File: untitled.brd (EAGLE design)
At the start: 92.9 x 80 mm, 176 parts, among them IC1 MCP23017SS, IC4 MCP23017SS, K2 351, Q1 S9013, U49 PC817X2NIP0F, X1 MSTBA12, X2 MSTBA12, X5 MSTBA3, X6 MSTBA3, X7 MSTBA2, X8 MSTBA2

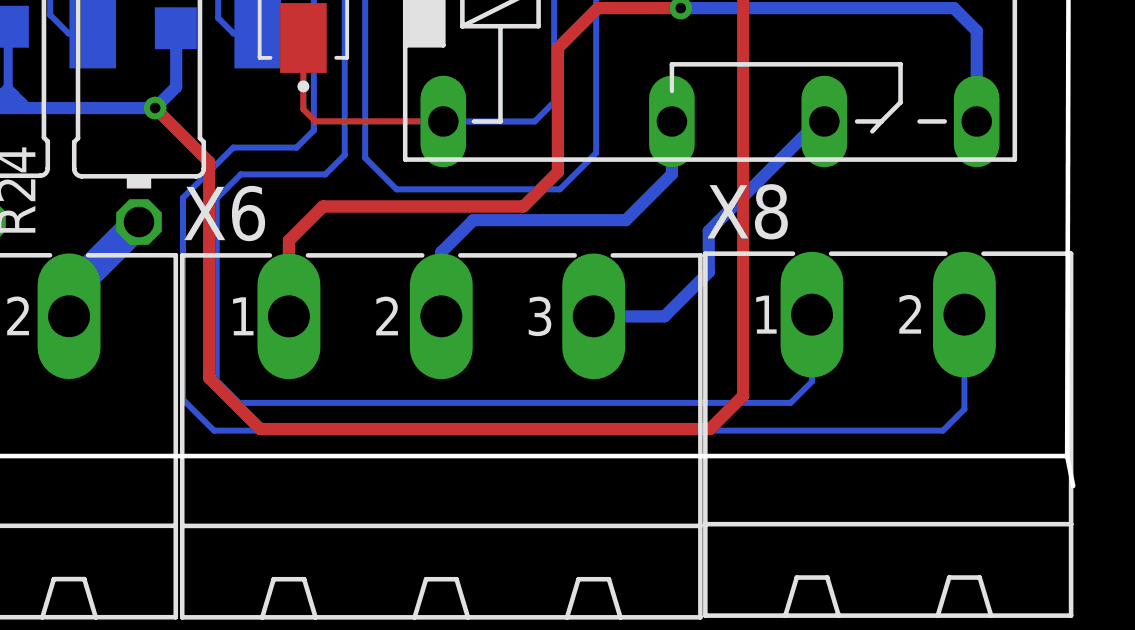
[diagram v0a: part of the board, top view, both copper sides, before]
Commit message: revisi .brd
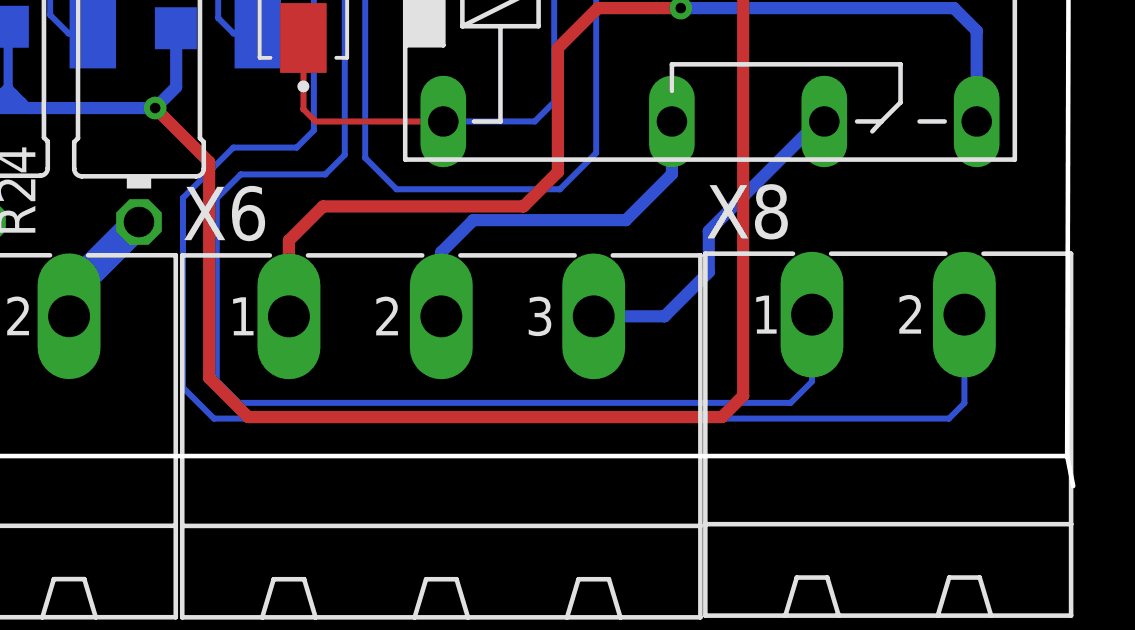
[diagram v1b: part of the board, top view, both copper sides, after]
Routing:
- net A+: track 56.6 -> 55.9 mm
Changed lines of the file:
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@@
 <wire x1="85.1" y1="24.6" x2="82.3" y2="21.8" width="0.4064" layer="1"/>
 <wire x1="82.3" y1="21.8" x2="82.3" y2="4.10525" width="0.4064" layer="1"/>
-<wire x1="82.3" y1="4.10525" x2="81.19475" y2="3" width="0.4064" layer="1"/>
-<wire x1="81.19475" y1="3" x2="66.2" y2="3" width="0.4064" layer="1"/>
-<wire x1="66.2" y1="3" x2="64.5" y2="4.7" width="0.4064" layer="1"/>
+<wire x1="82.3" y1="4.10525" x2="81.59475" y2="3.4" width="0.4064" layer="1"/>
+<wire x1="81.59475" y1="3.4" x2="65.8" y2="3.4" width="0.4064" layer="1"/>
+<wire x1="65.8" y1="3.4" x2="64.5" y2="4.7" width="0.4064" layer="1"/>
 <wire x1="64.5" y1="4.7" x2="64.5" y2="11.9" width="0.4064" layer="1"/>
 <wire x1="64.5" y1="11.9" x2="62.7" y2="13.7" width="0.4064" layer="1"/>
@@
 <contactref element="TTL-RS1" pad="A"/>
 <contactref element="X8" pad="2"/>
-<wire x1="89.6747" y1="6.81355" x2="89.6747" y2="3.66395" width="0.2" layer="16"/>
-<wire x1="89.6747" y1="3.66395" x2="88.95865" y2="2.9479" width="0.2" layer="16"/>
-<wire x1="88.95865" y1="2.9479" x2="64.66055" y2="2.9479" width="0.2" layer="16"/>
-<wire x1="64.66055" y1="2.9479" x2="63.627" y2="3.98145" width="0.2" layer="16"/>
-<wire x1="63.627" y1="3.98145" x2="63.627" y2="10.7061" width="0.2" layer="16"/>
+<wire x1="89.6747" y1="6.81355" x2="89.6747" y2="3.86395" width="0.2" layer="16"/>
+<wire x1="89.6747" y1="3.86395" x2="89.15865" y2="3.3479" width="0.2" layer="16"/>
+<wire x1="89.15865" y1="3.3479" x2="64.66055" y2="3.3479" width="0.2" layer="16"/>
+<wire x1="64.66055" y1="3.3479" x2="63.627" y2="4.38145" width="0.2" layer="16"/>
+<wire x1="63.627" y1="4.38145" x2="63.627" y2="10.7061" width="0.2" layer="16"/>
 <wire x1="63.627" y1="10.7061" x2="65.3034" y2="12.3825" width="0.2" layer="16"/>
 <wire x1="65.3034" y1="12.3825" x2="67.41795" y2="12.3825" width="0.2" layer="16"/>

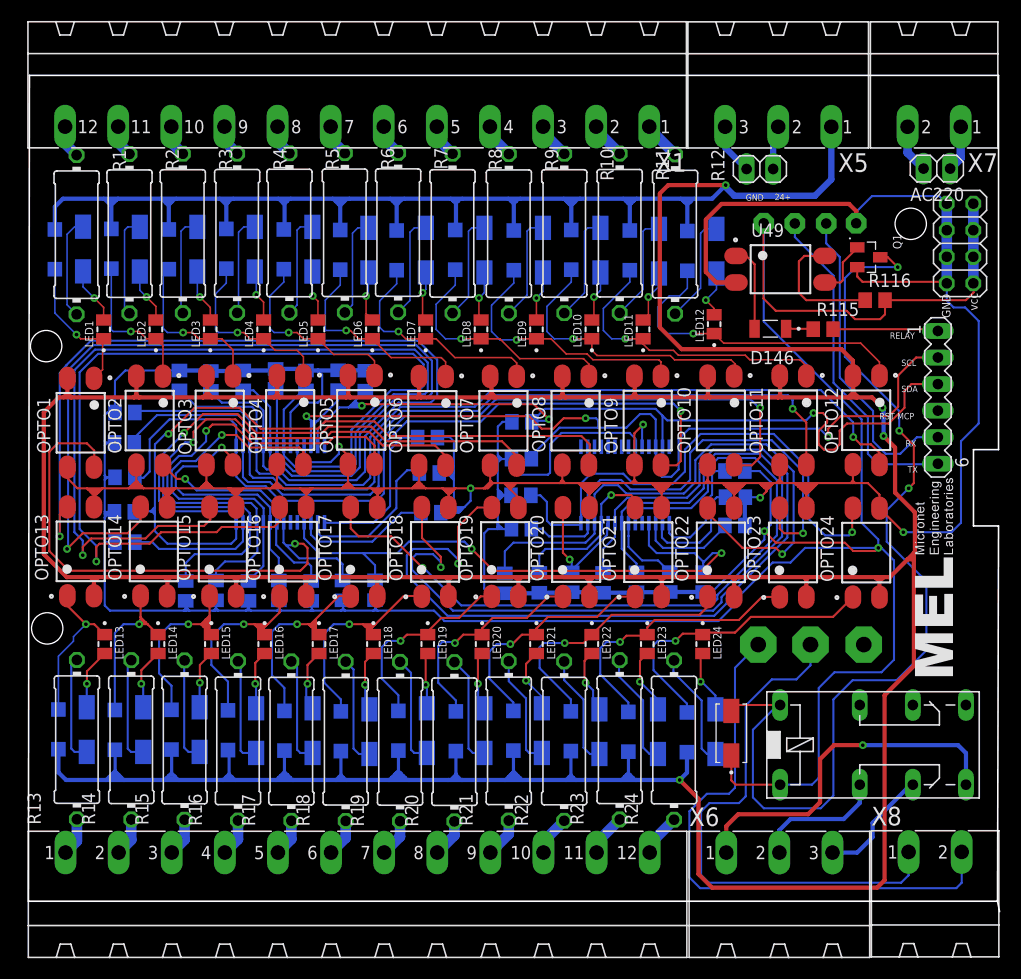
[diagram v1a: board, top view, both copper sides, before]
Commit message: revisi .brd
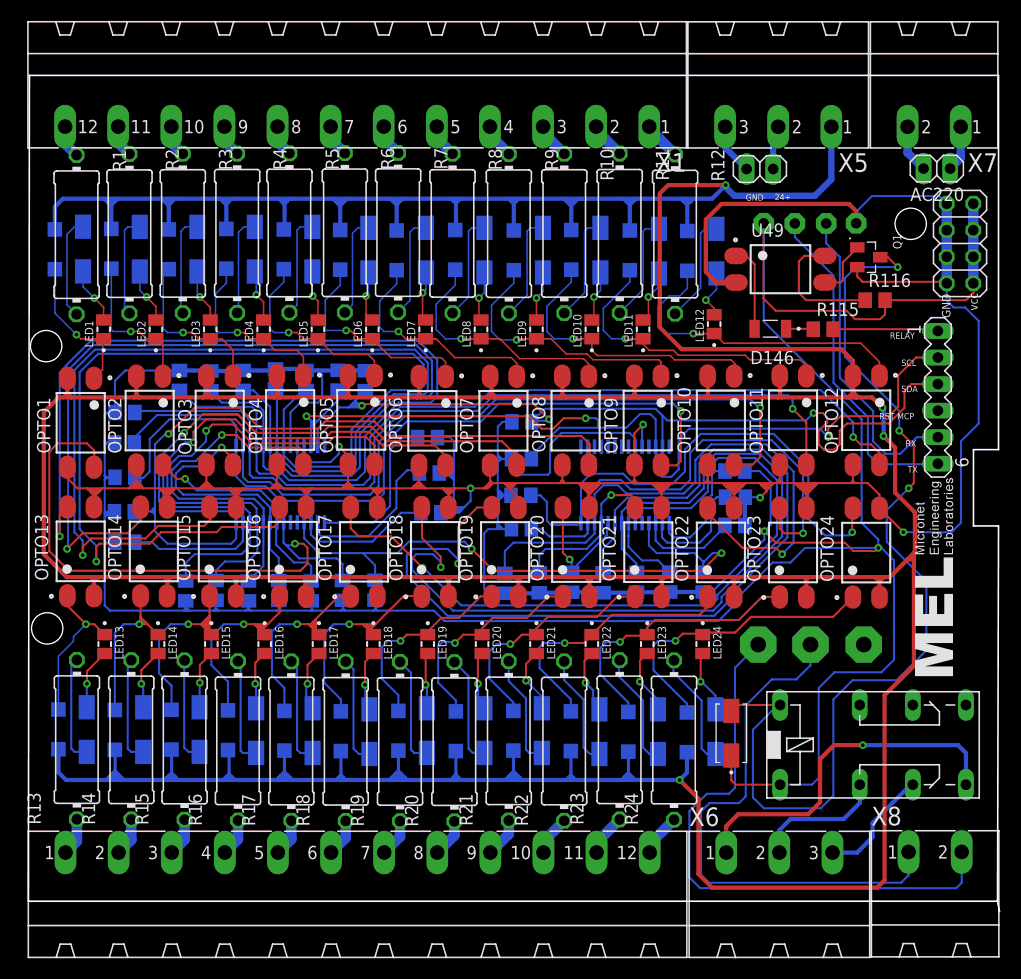
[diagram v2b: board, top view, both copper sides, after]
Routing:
- net GND: track 346.2 -> 345.5 mm
- net RELAY: track 10.7 -> 10.2 mm
